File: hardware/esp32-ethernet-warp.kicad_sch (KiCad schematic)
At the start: 52 parts, among them P101 FLASH, Q101 BC817, Q102 BC817, SW101 B3U-1000P, SW102 B3U-1000P, U101 TMP1075NDRLR, U103 PCF8523T, U104 ESP32-WROVER-E, U106 171010502, X101 32.768kHz

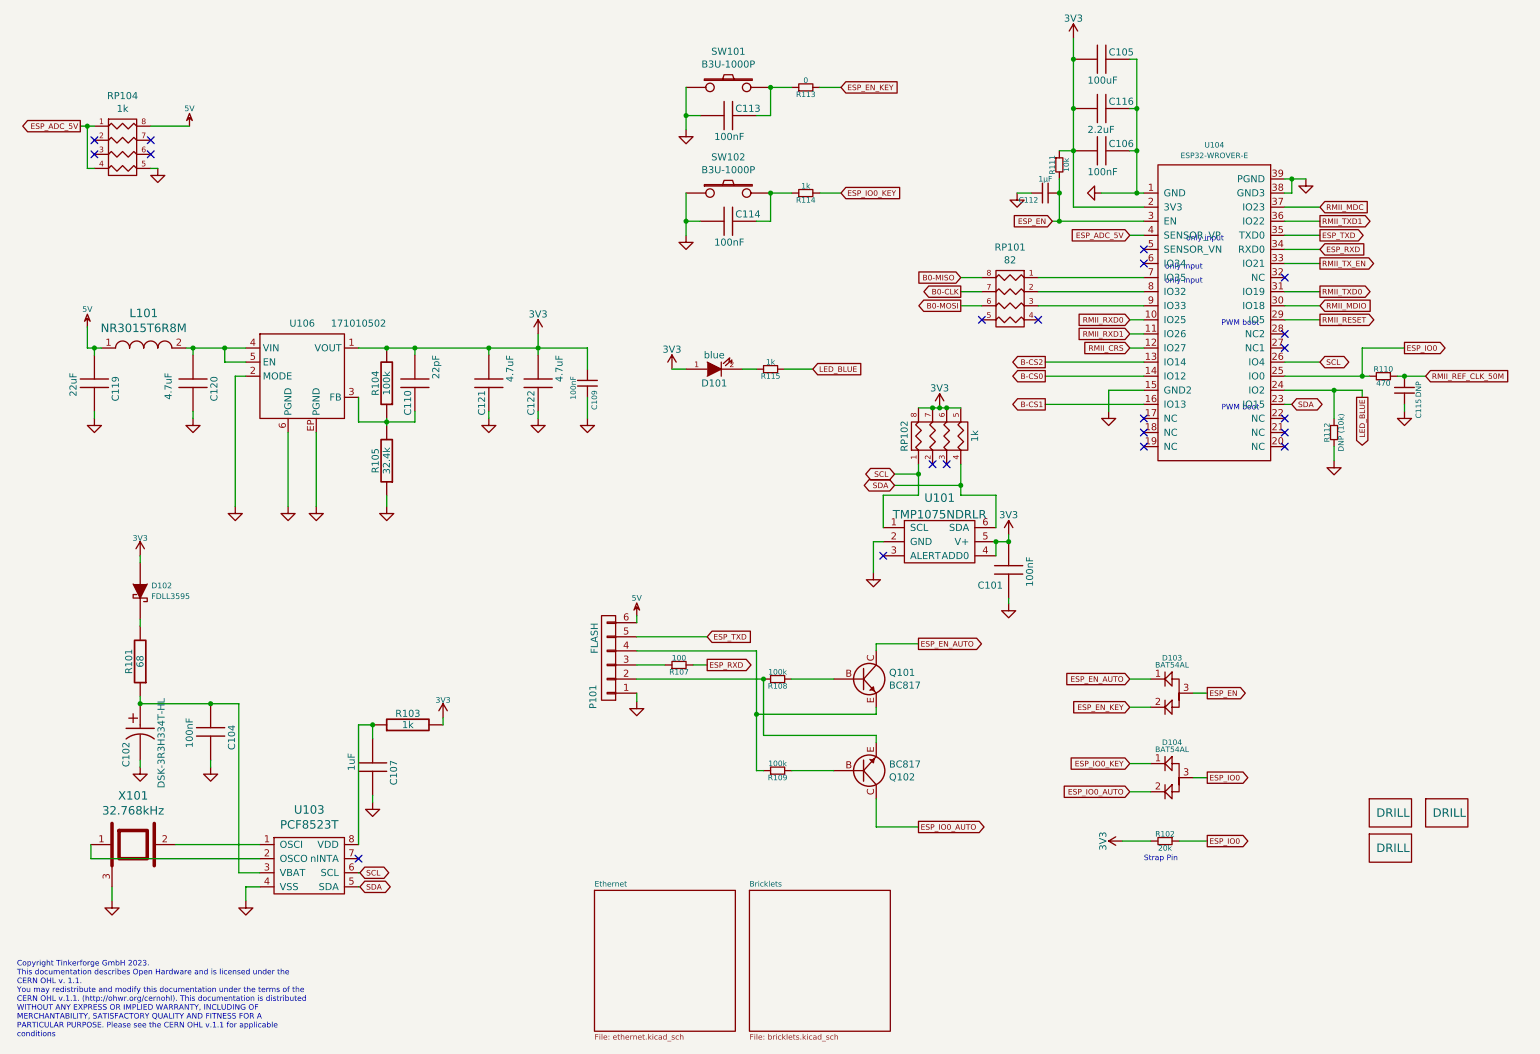
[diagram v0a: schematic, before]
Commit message: version 1.3 finished
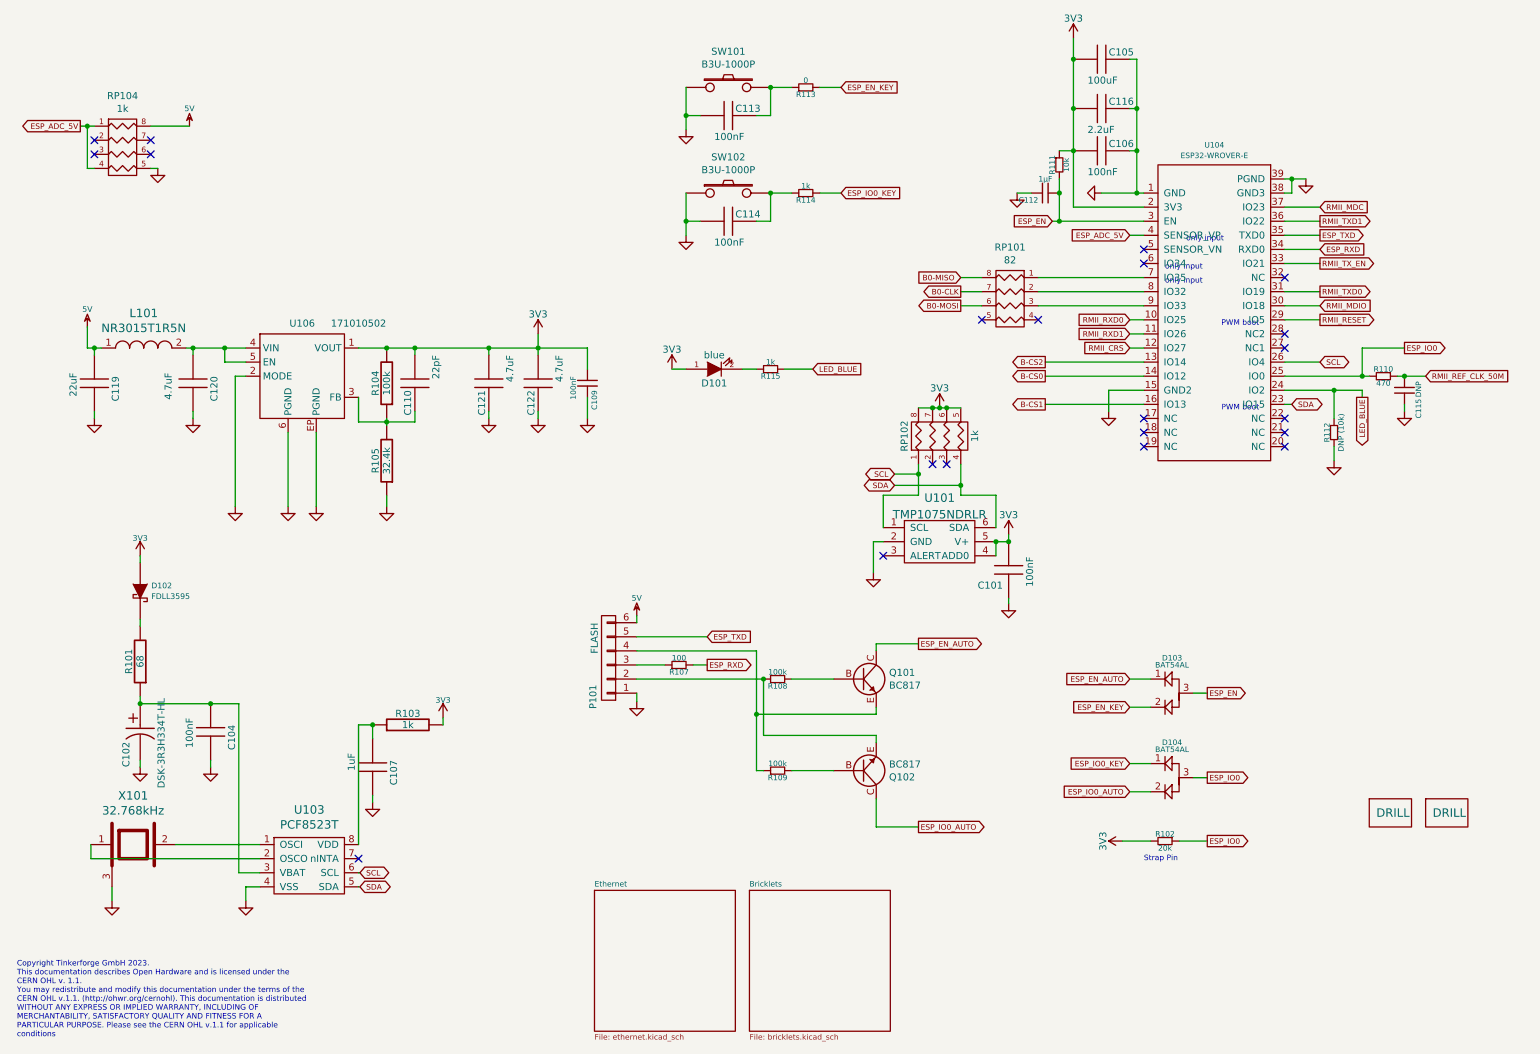
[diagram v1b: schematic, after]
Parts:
- removed F101: DRILL, kicad-libraries:LSMTSO-M3, symbol tinkerforge:DRILL
- L101: value NR3015T6R8M -> NR3015T1R5N

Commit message: Revert "version 1.3 finished"
This reverts commit c7f26ed94f03ba8104635e5142b3afb52f15755f.
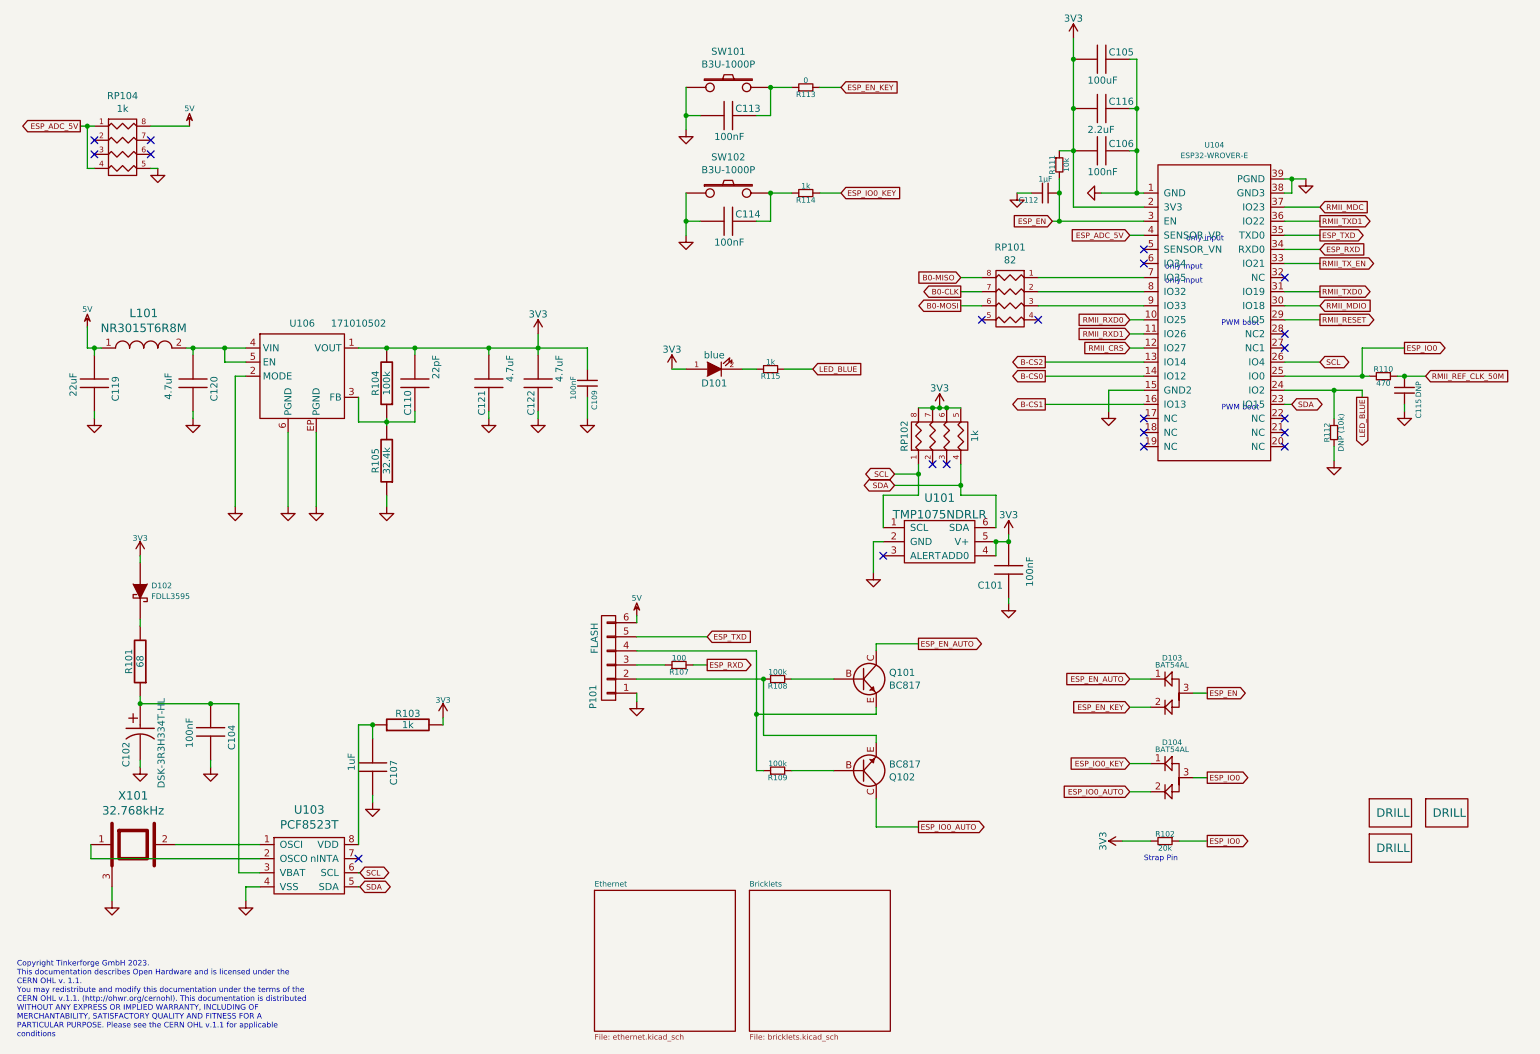
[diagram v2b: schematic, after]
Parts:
- added F101: DRILL, kicad-libraries:LSMTSO-M3, symbol tinkerforge:DRILL
- L101: value NR3015T1R5N -> NR3015T6R8M
